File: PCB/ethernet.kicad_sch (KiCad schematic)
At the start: 32 parts, among them J5 RJ45_Hanrun_HR911105A_Horizon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, SW2 SW_Push, U13 LAN8710A-EZC-TR, Y1 50MHz

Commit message: added basic capacitor footprints
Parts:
- C127, C128, C129, C131, C134: footprint (none) -> Capacitor_SMD:C_0402_1005Metric
- C140: footprint (none) -> Capacitor_SMD:C_0603_1608Metric
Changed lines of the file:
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@@
 			)
 		)
-		(property "Footprint" ""
+		(property "Footprint" "Capacitor_SMD:C_0402_1005Metric"
 			(at 72.0852 175.26 0)
 			(effects
@@
 			)
 		)
-		(property "Footprint" ""
+		(property "Footprint" "Capacitor_SMD:C_0402_1005Metric"
 			(at 286.7152 161.29 0)
 			(effects
@@
 			)
 		)
-		(property "Footprint" ""
+		(property "Footprint" "Capacitor_SMD:C_0402_1005Metric"
 			(at 167.3352 71.12 0)
 			(effects
@@
 			)
 		)
-		(property "Footprint" ""
+		(property "Footprint" "Capacitor_SMD:C_0402_1005Metric"
 			(at 154.6352 71.12 0)
 			(effects
@@
 			)
 		)
-		(property "Footprint" ""
+		(property "Footprint" "Capacitor_SMD:C_0402_1005Metric"
 			(at 126.6952 71.12 0)
 			(effects
@@
 			)
 		)
-		(property "Footprint" ""
+		(property "Footprint" "Capacitor_SMD:C_0603_1608Metric"
 			(at 158.4452 96.52 0)
 			(effects

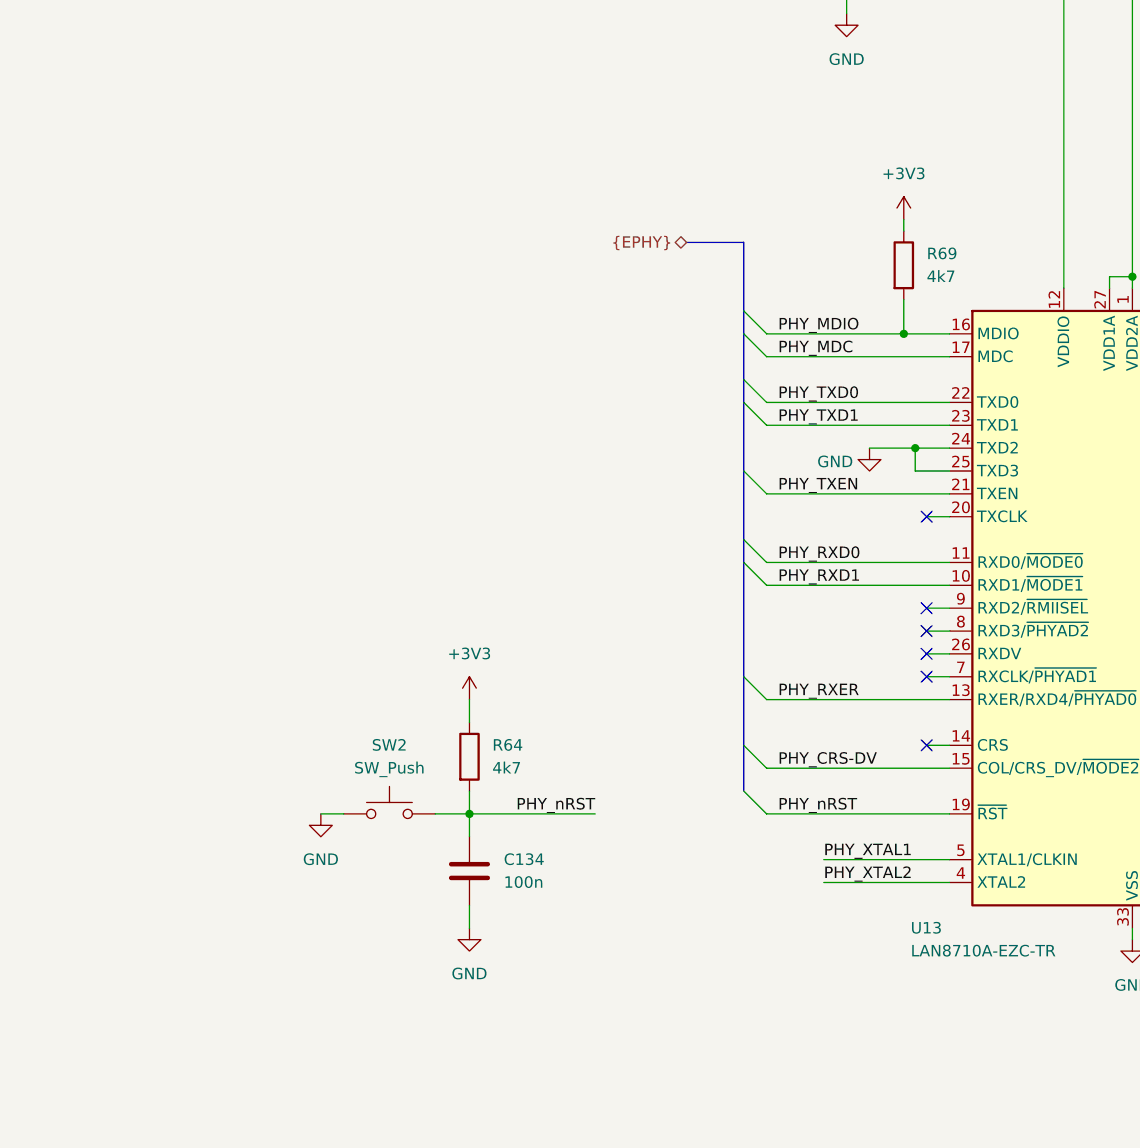
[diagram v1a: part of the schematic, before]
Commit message: cleaning up ethernet, added some dampening resistors
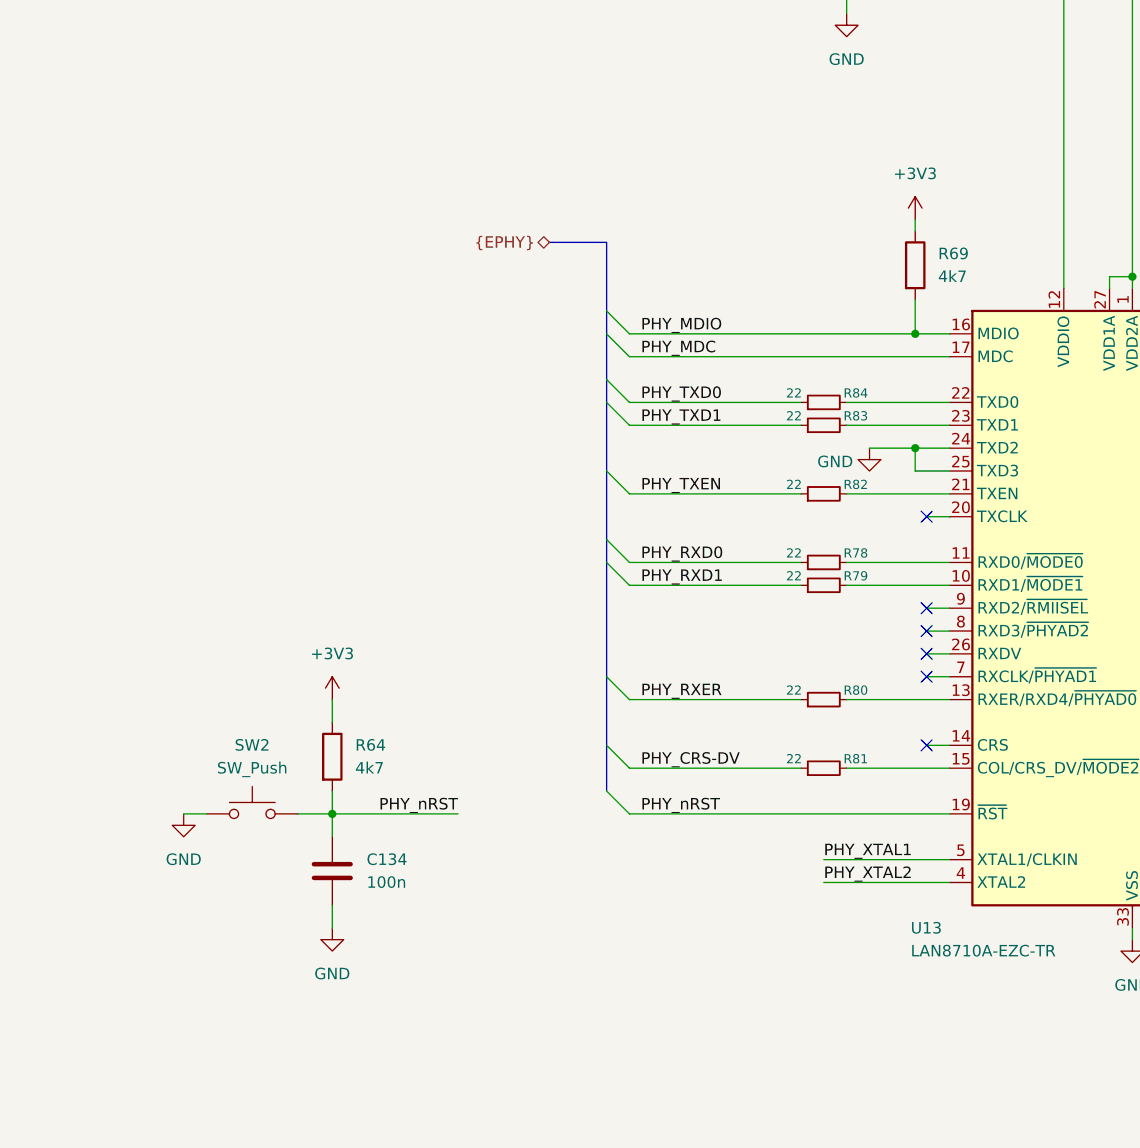
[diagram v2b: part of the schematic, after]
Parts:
- added R78, R79, R80, R81, R82, R83, R84: 22, symbol Device:R_Small
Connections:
- net PHY_CRS-DV: now also R81.1; no longer U13.15 (COL/CRS_DV/~{MODE2})
- net PHY_RXD0: now also R78.1; no longer U13.11 (RXD0/~{MODE0})
- net PHY_RXD1: now also R79.1; no longer U13.10 (RXD1/~{MODE1})
- net PHY_RXER: now also R80.1; no longer U13.13 (RXER/RXD4/~{PHYAD0})
- net PHY_TXD0: now also R84.1; no longer U13.22 (TXD0)
- net PHY_TXD1: now also R83.1; no longer U13.23 (TXD1)
- net PHY_TXEN: now also R82.1; no longer U13.21 (TXEN)
- new net: R79.2, U13.10 (RXD1/~{MODE1})
- new net: R81.2, U13.15 (COL/CRS_DV/~{MODE2})
- new net: R83.2, U13.23 (TXD1)
- new net: R82.2, U13.21 (TXEN)
- new net: R84.2, U13.22 (TXD0)
- new net: R78.2, U13.11 (RXD0/~{MODE0})
- new net: R80.2, U13.13 (RXER/RXD4/~{PHYAD0})
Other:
- moved on the sheet: C134, R64, R69, SW2
